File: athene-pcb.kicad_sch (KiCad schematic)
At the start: 152 parts, among them J1 HRO-TYPE-C-31-M-12, K1 KEYSW, K10 KEYSW, K11 KEYSW, K12 KEYSW, K13 KEYSW, K14 KEYSW, K15 KEYSW, K16 KEYSW, K17 KEYSW, K18 KEYSW, K19 KEYSW, K2 KEYSW, K20 KEYSW, K21 KEYSW, K22 KEYSW, K23 KEYSW, K24 KEYSW, K25 KEYSW, K26 KEYSW, K27 KEYSW, K28 KEYSW, K29 KEYSW, K3 KEYSW, K30 KEYSW, K31 KEYSW, K32 KEYSW, K33 KEYSW, K34 KEYSW, K35 KEYSW, K36 KEYSW, K37 KEYSW, K38 KEYSW, K39 KEYSW, K4 KEYSW, K40 KEYSW, K41 KEYSW, K42 KEYSW, K43 KEYSW, K44 KEYSW, K45 KEYSW, K46 KEYSW, K47 KEYSW, K48 KEYSW, K49 KEYSW, K5 KEYSW, K50 KEYSW, K51 KEYSW, K52 KEYSW, K53 KEYSW, K54 KEYSW, K55 KEYSW, K56 KEYSW, K57 KEYSW, K58 KEYSW, K59 KEYSW, K6 KEYSW, K60 KEYSW, K61 KEYSW, K62 KEYSW, K63 KEYSW, K64 KEYSW, K65 KEYSW, K66 KEYSW, K67 KEYSW, K7 KEYSW, K8 KEYSW, K9 KEYSW, U1 ATmega32U4-AU, U2 USBLC6-2SC6, Y1 16MHz

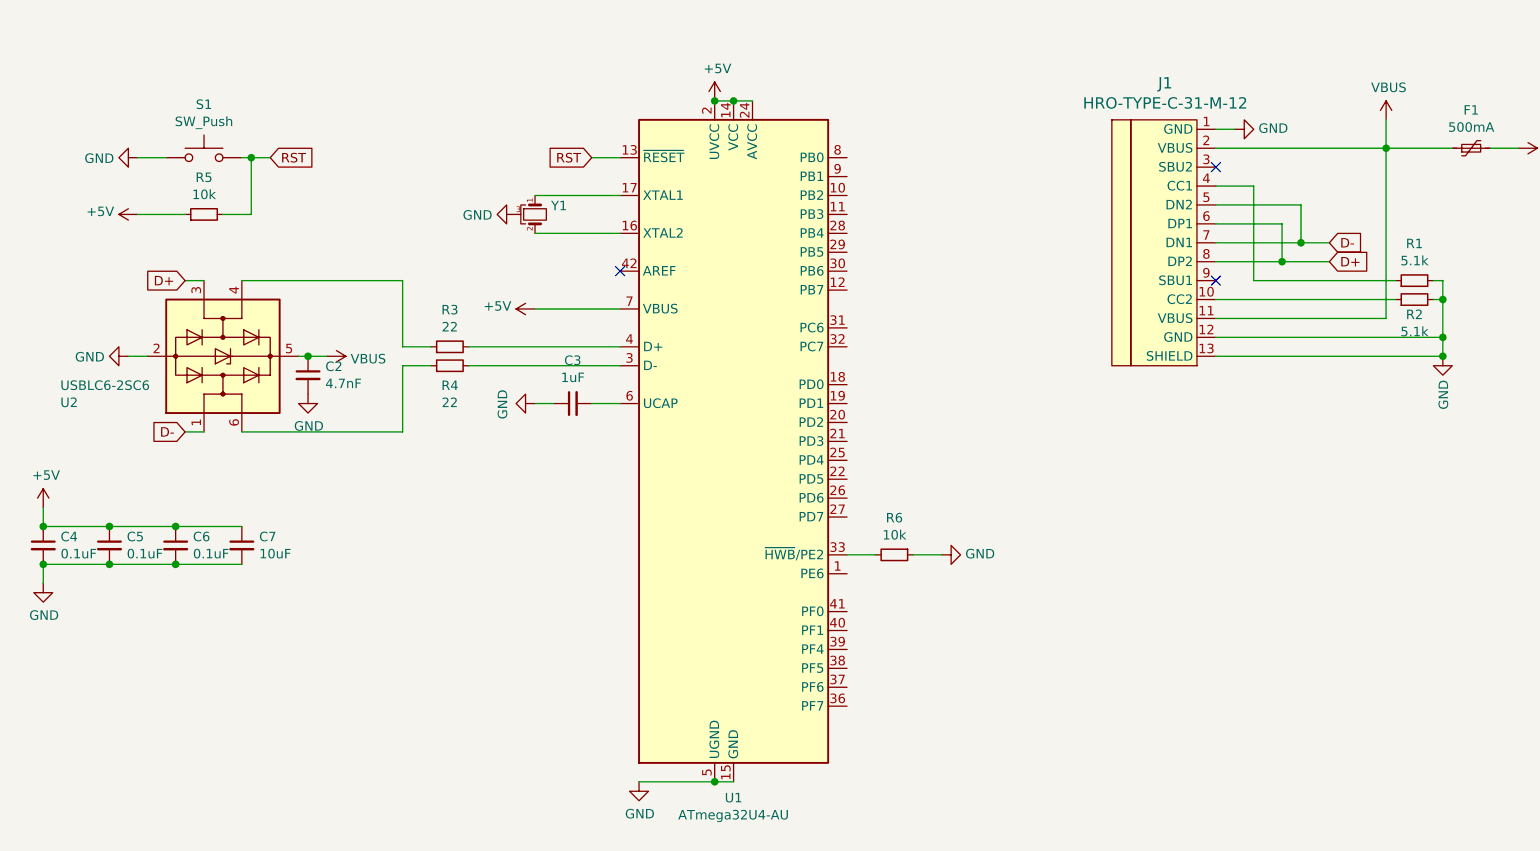
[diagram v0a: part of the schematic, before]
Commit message: v1 ready for review
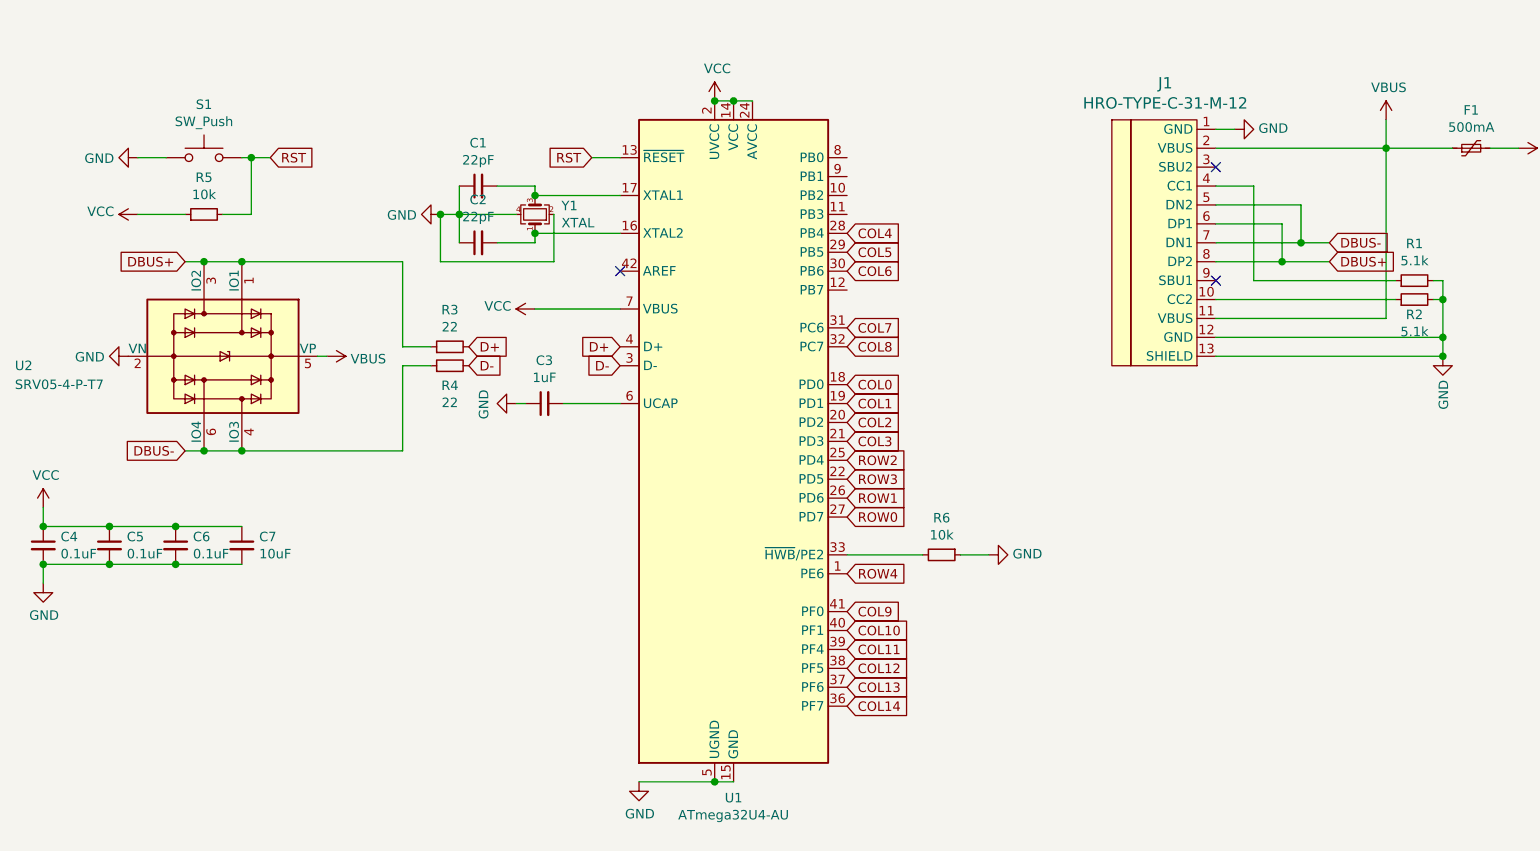
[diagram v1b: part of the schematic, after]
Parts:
- removed Y1: 16MHz, Crystal:Resonator_SMD_muRata_CSTxExxV-3Pin_3.0x1.1mm, symbol Device:Crystal_GND3_Small
- added C1: 22pF, Capacitor_SMD:C_0805_2012Metric, symbol Device:C_Small
- added Y1: XTAL, Crystal:Crystal_SMD_3225-4Pin_3.2x2.5mm, symbol Device:Crystal_GND24_Small
- C2: value 4.7nF -> 22pF
- D31: value b -> D
- K1, K10, K11, K12, K13, K14, K15, K16, K17, K18, K19, K2, K20, K21, K22, K23, K24, K25, K26, K27, K28, K29, K3, K30, K31, K32, K33, K34, K35, K36, K37, K38, K39, K4, K40, K41, K42, K43, K44, K45, K46, K47, K48, K49, K5, K50, K51, K52, K53, K54, K55, K56, K57, K58, K59, K6, K60, K61, K62, K63, K64, K65, K66, K67, K7, K8, K9: footprint keyboard_parts:Kailh_MX_Socket_LED -> keyboard_parts:Kailh_MX_Socket (3D)
- U2: value USBLC6-2SC6 -> SRV05-4-P-T7; symbol Power_Protection:USBLC6-2SC6 -> Power_Protection:SRV05-4
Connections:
- net +5V is gone; now on net VCC: C4.1, C5.1, C6.1, C7.1, R5.1, U1.14 (VCC), U1.2 (UVCC), U1.24 (AVCC), U1.34 (VCC), U1.44 (AVCC), U1.7 (VBUS)
- net COL0: now also U1.18 (PD0)
- net COL1: now also U1.19 (PD1)
- net COL10: now also U1.40 (PF1)
- net COL11: now also U1.39 (PF4)
- net COL12: now also U1.38 (PF5)
- net COL13: now also U1.37 (PF6)
- net COL14: now also U1.36 (PF7)
- net COL2: now also U1.20 (PD2)
- net COL3: now also U1.21 (PD3)
- net COL4: now also U1.28 (PB4)
- net COL5: now also U1.29 (PB5)
- net COL6: now also U1.30 (PB6)
- net COL7: now also U1.31 (PC6)
- net COL8: now also U1.32 (PC7)
- net COL9: now also U1.41 (PF0)
- net D+: now also R3.2, U1.4 (D+); no longer J1.6 (DP1), J1.8 (DP2), U2.3 (I/O2)
- net D-: now also R4.2, U1.3 (D-); no longer J1.5 (DN2), J1.7 (DN1), U2.1 (I/O1)
- net GND: now also C2.1, C1.1, Y1.2, Y1.4; no longer C2.2
- net ROW0: now also U1.27 (PD7)
- net ROW1: now also U1.26 (PD6)
- net ROW2: now also U1.25 (PD4)
- net ROW3: now also U1.22 (PD5)
- net ROW4: now also U1.1 (PE6)
- net VBUS: no longer C2.1
- net DBUS+: now reaches R3.1
- net DBUS+: now also J1.6 (DP1), J1.8 (DP2), U2.1 (IO1), U2.3 (IO2); no longer U2.4 (I/O2)
- net DBUS-: now reaches R4.1, U2.6 (IO4)
- net DBUS-: now also J1.5 (DN2), J1.7 (DN1), U2.4 (IO3)
- net at U1.16 (XTAL2): now also C2.2, Y1.1
- net at U1.17 (XTAL1): now also C1.2, Y1.3
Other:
- moved on the sheet: C3, R6

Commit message: v1.0a update
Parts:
- added C10, C11, C12, C13, C14, C15, C9: 0.1uF, Capacitor_SMD:C_0805_2012Metric, symbol Device:C_Small
- added C8: 4.7nF, Capacitor_SMD:C_0805_2012Metric, symbol Device:C_Small
- added J2: AVR-ISP-6, random-keyboard-parts:Reset_Pretty-Mask, symbol Connector:AVR-ISP-6
- added R7: 1M, Resistor_SMD:R_0805_2012Metric, symbol Device:R_Small
- added RGB1, RGB2, RGB3, RGB4, RGB5, RGB6, RGB7: SK6812, LED_SMD:LED_SK6812_PLCC4_5.0x5.0mm_P3.2mm, symbol LED:SK6812
- K29, K37, K60, K66: footprint keyboard_parts:Kailh_MX_Socket (3D) -> keyboard_parts:Kailh_MX_Socket (3D) 1_Circle
- renumbered C6 to C5, C5 to C6
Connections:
- net COL10: now also U1.37 (PF6); no longer U1.40 (PF1)
- net COL11: now also U1.38 (PF5); no longer U1.39 (PF4)
- net COL12: now also U1.39 (PF4); no longer U1.38 (PF5)
- net COL13: now also U1.40 (PF1); no longer U1.37 (PF6)
- net COL14: now also U1.41 (PF0); no longer U1.36 (PF7)
- net COL9: now also U1.36 (PF7); no longer U1.41 (PF0)
- net GND: now also C10.2, C11.2, C12.2, C13.2, C14.2, C15.2, C8.2, C9.2, J2.6 (GND), R7.1, RGB1.1 (VSS), RGB2.1 (VSS), RGB3.1 (VSS), RGB4.1 (VSS), RGB5.1 (VSS), RGB6.1 (VSS), RGB7.1 (VSS); no longer J1.13 (SHIELD)
- net ROW0: now also U1.25 (PD4); no longer U1.27 (PD7)
- net ROW2: now also U1.27 (PD7); no longer U1.25 (PD4)
- net RST: now also J2.5 (~RST)
- net VCC: now also C10.1, C11.1, C12.1, C13.1, C14.1, C15.1, C9.1, J2.2 (VCC), RGB1.3 (VDD), RGB2.3 (VDD), RGB3.3 (VDD), RGB4.3 (VDD), RGB5.3 (VDD), RGB6.3 (VDD), RGB7.3 (VDD)
- net MOSI: now reaches U1.10 (PB2)
- net MOSI: now also J2.4 (MOSI)
- net MISO: now reaches U1.11 (PB3)
- net MISO: now also J2.1 (MISO)
- net RGB: now reaches U1.12 (PB7)
- net RGB: now also RGB1.2 (DIN)
- net SCLK: now reaches U1.9 (PB1)
- net SCLK: now also J2.3 (SCK)
- new net: C8.1, J1.13 (SHIELD), R7.2
- new net: RGB1.4 (DOUT), RGB2.2 (DIN)
- new net: RGB2.4 (DOUT), RGB3.2 (DIN)
- new net: RGB6.4 (DOUT), RGB7.2 (DIN)
- new net: RGB3.4 (DOUT), RGB4.2 (DIN)
- new net: RGB4.4 (DOUT), RGB5.2 (DIN)
- new net: RGB5.4 (DOUT), RGB6.2 (DIN)
- no-connect marks 3 -> 4
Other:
- note added: "DECOUPLING CAPACITORS"
- note added: "ESD"
- note added: "ISP"
- note added: "MICROCONTROLLER UNIT"
- note added: "RESET"
- note added: "RGB UNDERGLOW"
- note added: "SWITCH MATRIX"
- note added: "USB-C CONNECTOR"
- moved on the sheet: C1, C2, C3, C4, C5, C6, C7, D1, D10, D11, D12, D13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
